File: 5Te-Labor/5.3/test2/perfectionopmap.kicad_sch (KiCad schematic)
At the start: 7 parts, among them U1 4023, U2 4023, U3 4013

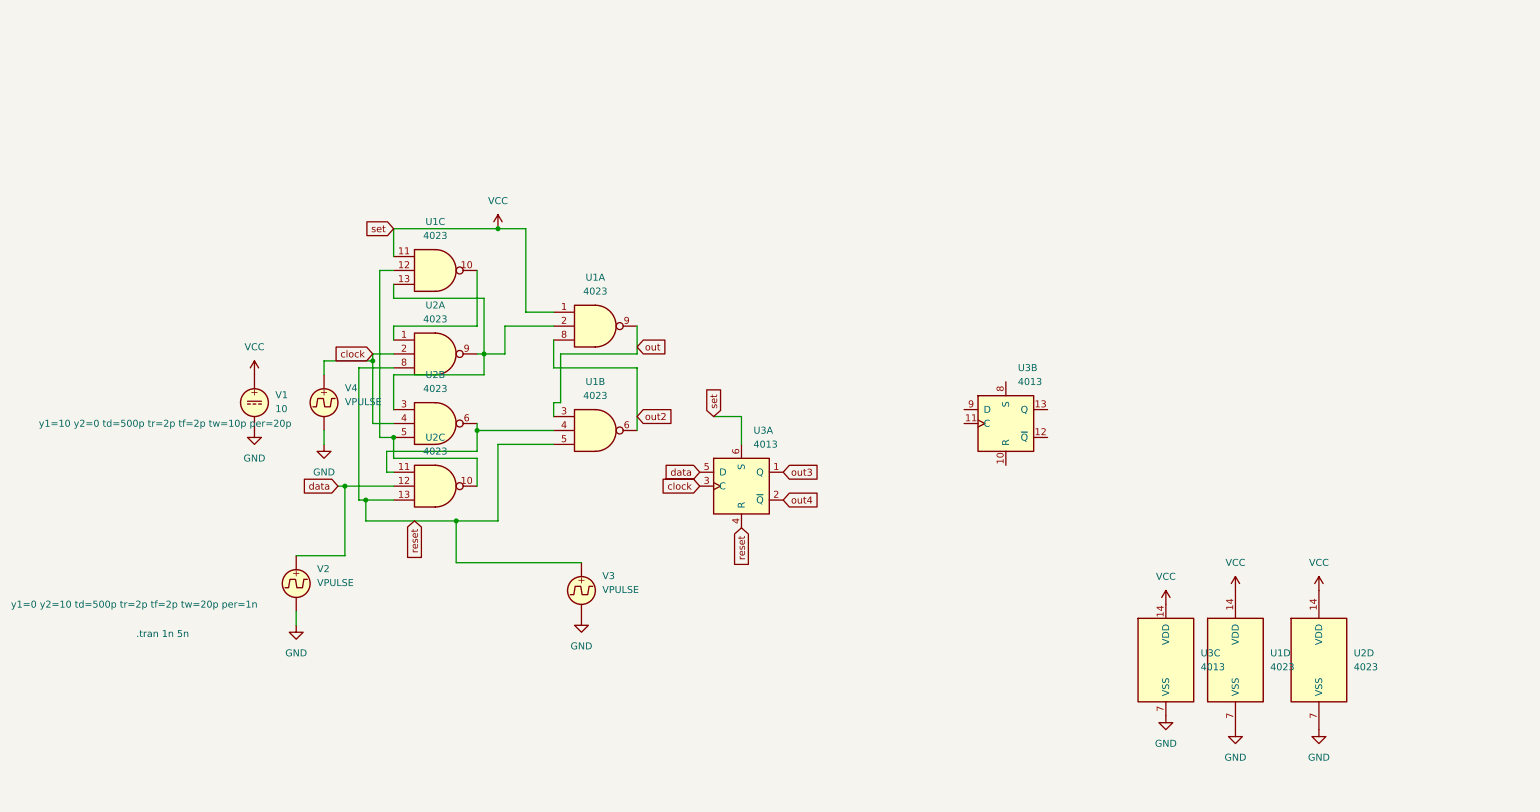
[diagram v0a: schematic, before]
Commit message: an attempt was made
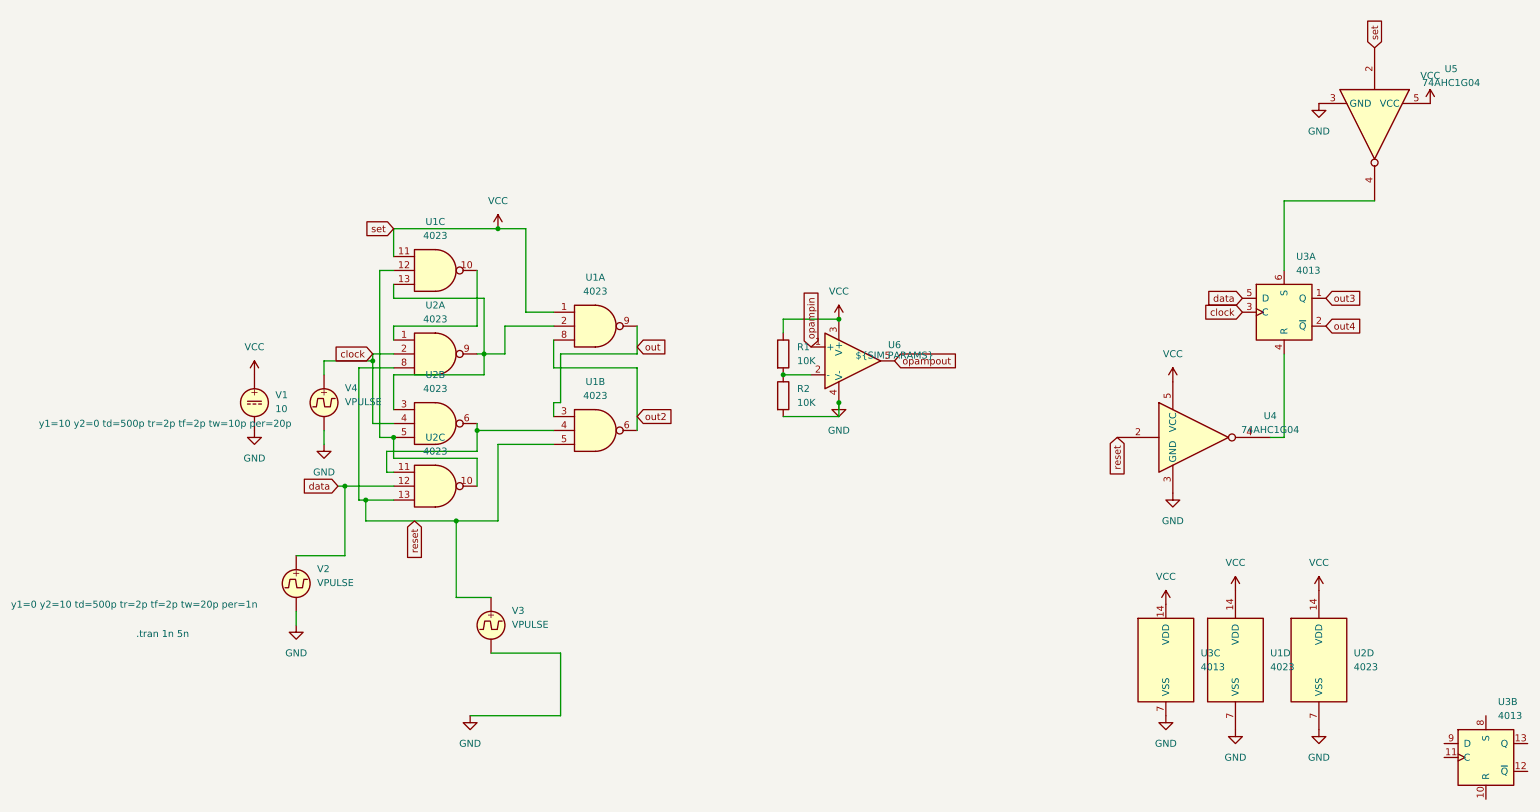
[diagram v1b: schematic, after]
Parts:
- added R1, R2: 10K, symbol Device:R
- added U4, U5: 74AHC1G04, symbol 74xGxx:74AHC1G04
- added U6: ${SIM.PARAMS}, symbol Simulation_SPICE:OPAMP
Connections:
- net GND: now also R2.2, U4.3 (GND), U5.3 (GND), U6.4 (V-)
- net VCC: now also R1.1, U4.5 (VCC), U5.2, U5.5 (VCC), U6.3 (V+); no longer U3.6 (S)
- net reset: now also U4.2; no longer U3.4 (R)
- new net: R1.2, R2.1, U6.2 (-)
- new net: U3.4 (R), U4.4
- new net: U3.6 (S), U5.4
- new net opampin: U6.1 (+)
- new net opampout: U6.5
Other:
- moved on the sheet: U3A, U3B, V3
